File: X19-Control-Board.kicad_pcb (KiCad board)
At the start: 2 copper layers, 100 x 100 mm, 0 parts

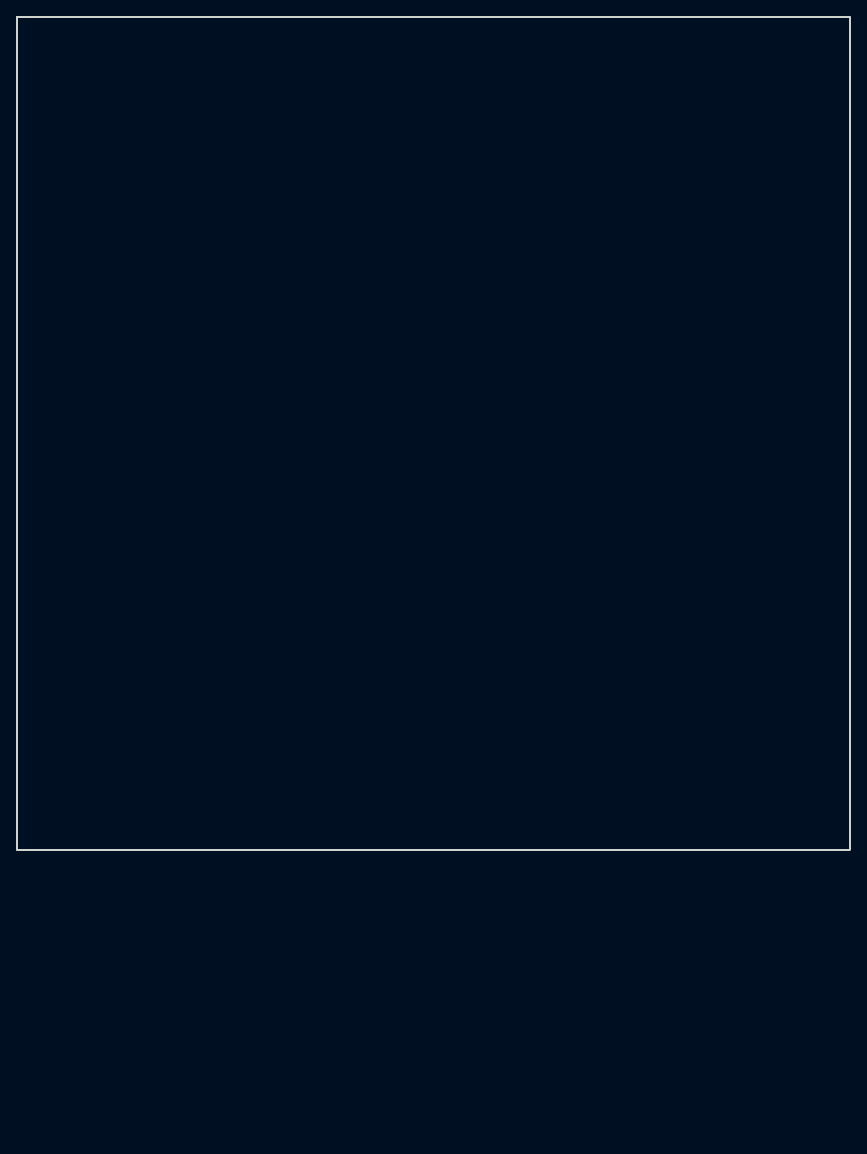
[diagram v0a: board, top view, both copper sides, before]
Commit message: We are BACK
I am feeling myself. Lots of progress here.
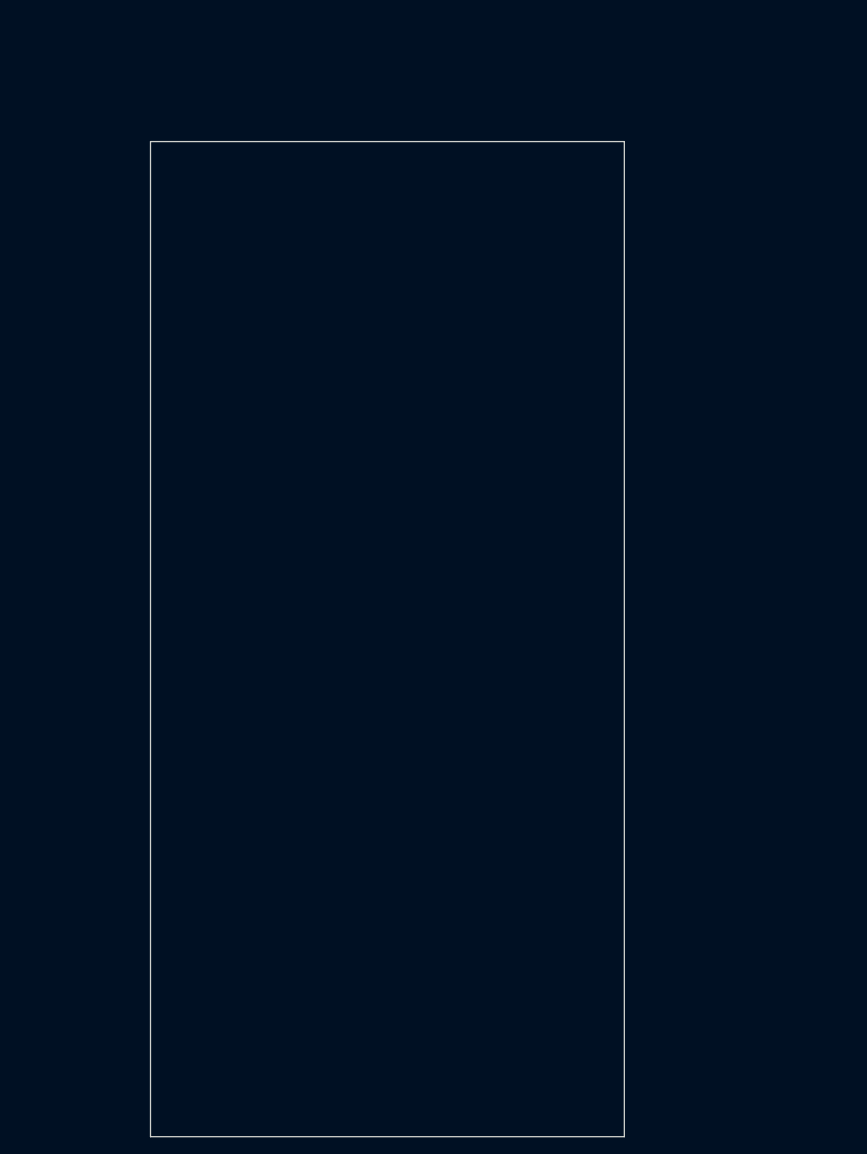
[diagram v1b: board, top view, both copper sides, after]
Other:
- board size 100 x 100 mm -> 56.9 x 119.5 mm
- copper layers 2 -> 4
- board text added: "Check board Dim"
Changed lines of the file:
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@@
 	)
 	(layers
-		(0 "F.Cu" signal)
-		(2 "B.Cu" signal)
+		(0 "F.Cu" signal "SIG1")
+		(4 "In1.Cu" signal "GND")
+		(6 "In2.Cu" signal "3.3-12V SPLIT PWR")
+		(2 "B.Cu" signal "SIG2")
 		(9 "F.Adhes" user "F.Adhesive")
 		(11 "B.Adhes" user "B.Adhesive")
@@
 	)
 	(setup
+		(stackup
+			(layer "F.SilkS"
+				(type "Top Silk Screen")
+			)
+			(layer "F.Paste"
+				(type "Top Solder Paste")
+			)
+			(layer "F.Mask"
+				(type "Top Solder Mask")
+				(thickness 0.01)
+			)
+			(layer "F.Cu"
+				(type "copper")
+				(thickness 0.035)
+			)
+			(layer "dielectric 1"
+				(type "prepreg")
+				(thickness 0.1)
+				(material "FR4")
+				(epsilon_r 4.5)
+				(loss_tangent 0.02)
+			)
+			(layer "In1.Cu"
+				(type "copper")
+				(thickness 0.035)
+			)
+			(layer "dielectric 2"
+				(type "core")
+				(thickness 1.24)
+				(material "FR4")
+				(epsilon_r 4.5)
+				(loss_tangent 0.02)
+			)
+			(layer "In2.Cu"
+				(type "copper")
+				(thickness 0.035)
+			)
+			(layer "dielectric 3"
+				(type "prepreg")
+				(thickness 0.1)
+				(material "FR4")
+				(epsilon_r 4.5)
+				(loss_tangent 0.02)
+			)
+			(layer "B.Cu"
+				(type "copper")
+				(thickness 0.035)
+			)
+			(layer "B.Mask"
+				(type "Bottom Solder Mask")
+				(thickness 0.01)
+			)
+			(layer "B.Paste"
+				(type "Bottom Solder Paste")
+			)
+			(layer "B.SilkS"
+				(type "Bottom Silk Screen")
+			)
+			(copper_finish "None")
+			(dielectric_constraints no)
+		)
 		(pad_to_mask_clearance 0)
 		(allow_soldermask_bridges_in_footprints no)
@@
 		(capping no)
 		(filling no)
+		(zone_defaults)
 		(pcbplotparams
 			(layerselection 0x00000000_00000000_55555555_5755f5ff)
@@
 		)
 	)
-	(gr_rect (start 0 0) (end 100 100)
-		(stroke (width 0.1) (type solid))
-		(fill none)
+	(gr_rect
+		(start 16.0234 14.9514)
+		(end 72.9234 134.4514)
+		(stroke
+			(width 0.05)
+			(type solid)
+		)
+		(fill no)
 		(layer "Edge.Cuts")
 	)
-	(gr_rect (start 0 0) (end 100 100)
-		(stroke (width 0.1) (type solid))
-		(fill none)
-		(layer "Edge.Cuts")
+	(gr_text "Check board Dim"
+		(at -10.3378 76.708 0)
+		(layer "User.1")
+		(effects
+			(font
+				(size 1 1)
+				(thickness 0.15)
+			)
+			(justify left bottom)
+		)
 	)
 	(embedded_fonts no)
-	(gr_rect (start 0 0) (end 100 100) (layer "Edge.Cuts")
-		(stroke (width 0.1) (type solid))
-		(fill none)
-	)
 )
